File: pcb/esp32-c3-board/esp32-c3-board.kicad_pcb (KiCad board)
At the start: 2 copper layers, 118.7 x 40.6 mm, 30 parts, among them P101 CAN, P102 RS485, P3 CONN_1, P4 CONN_1, P5 CONN_1, P6 CONN_1, U102 TJA1050, U2 esp32-c3-ebay, U4 6N137, U5 DCDCConverter, U6 6N137

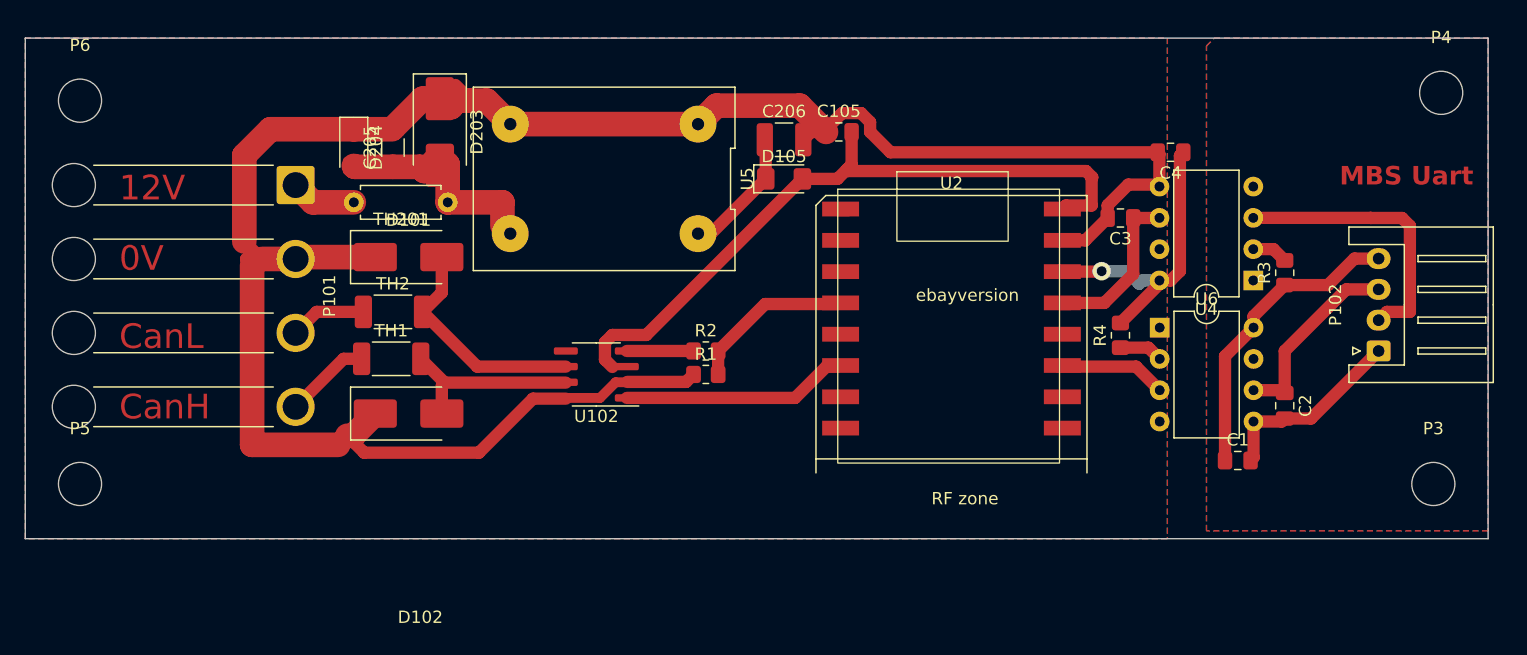
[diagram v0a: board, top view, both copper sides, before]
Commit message: Updated boards and readme
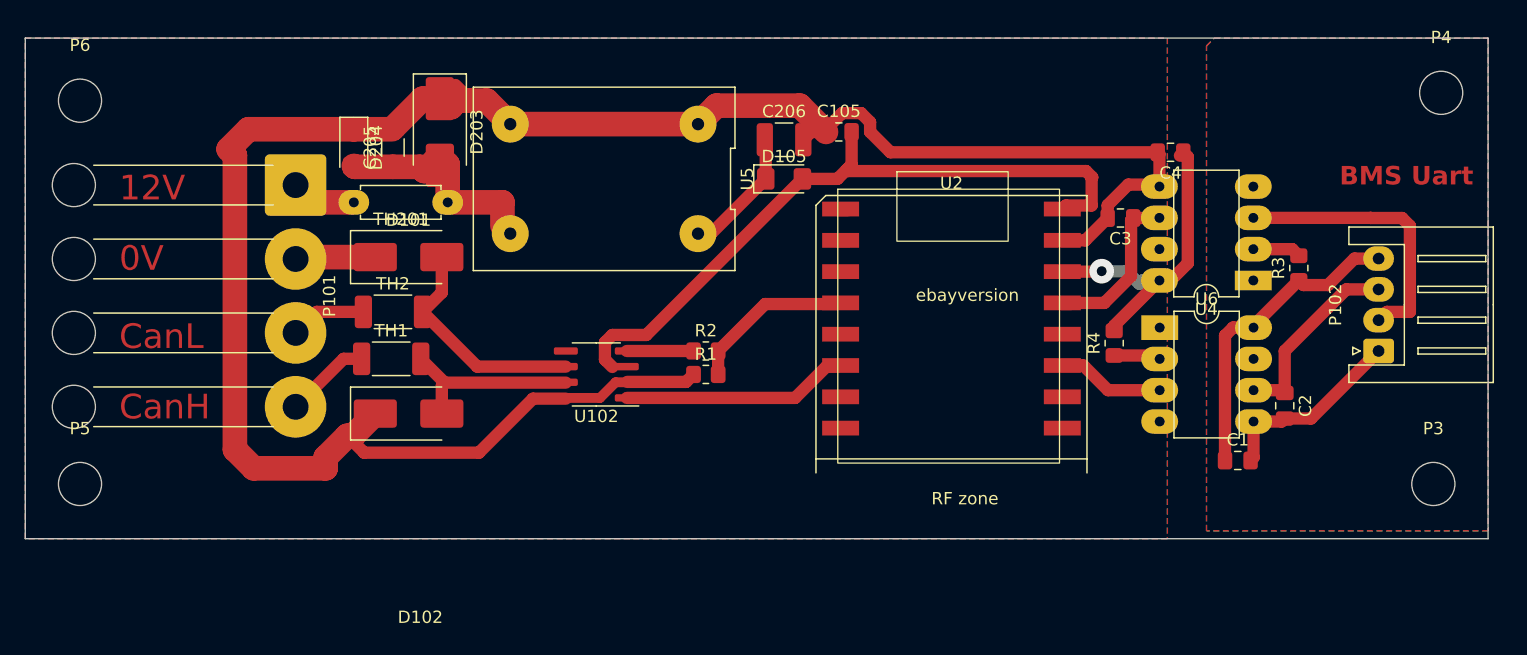
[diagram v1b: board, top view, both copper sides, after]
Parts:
- moved R3 1.20 mm to (116.1, 58.7)
- moved R4 0.81 mm to (101.1, 64.8)
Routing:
- net 3v3: track 24.9 -> 26.8 mm
- net GND: track 177.3 -> 176.3 mm
- net Net-(U4-A): track 2.93 -> 3.91 mm
- net 5V BMS: track 24.8 -> 25.6 mm
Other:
- board text added: "BMS Uart"
- board text removed: "MBS Uart"
